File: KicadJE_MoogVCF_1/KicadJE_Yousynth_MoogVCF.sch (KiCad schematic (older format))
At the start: 50 parts

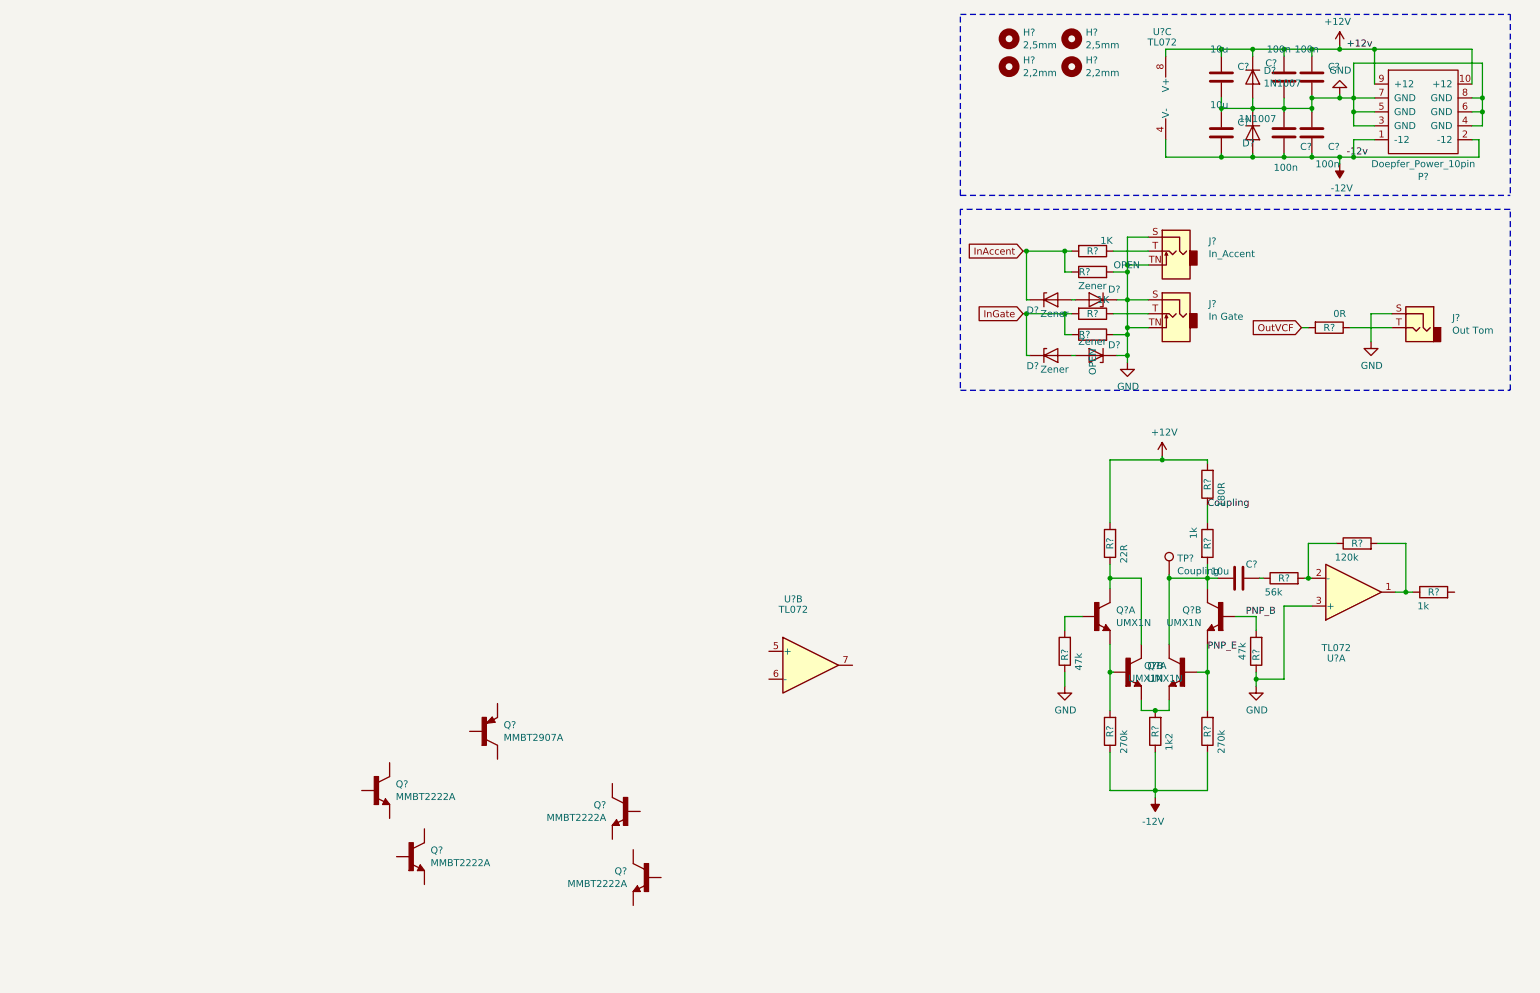
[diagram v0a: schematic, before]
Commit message: Footprints
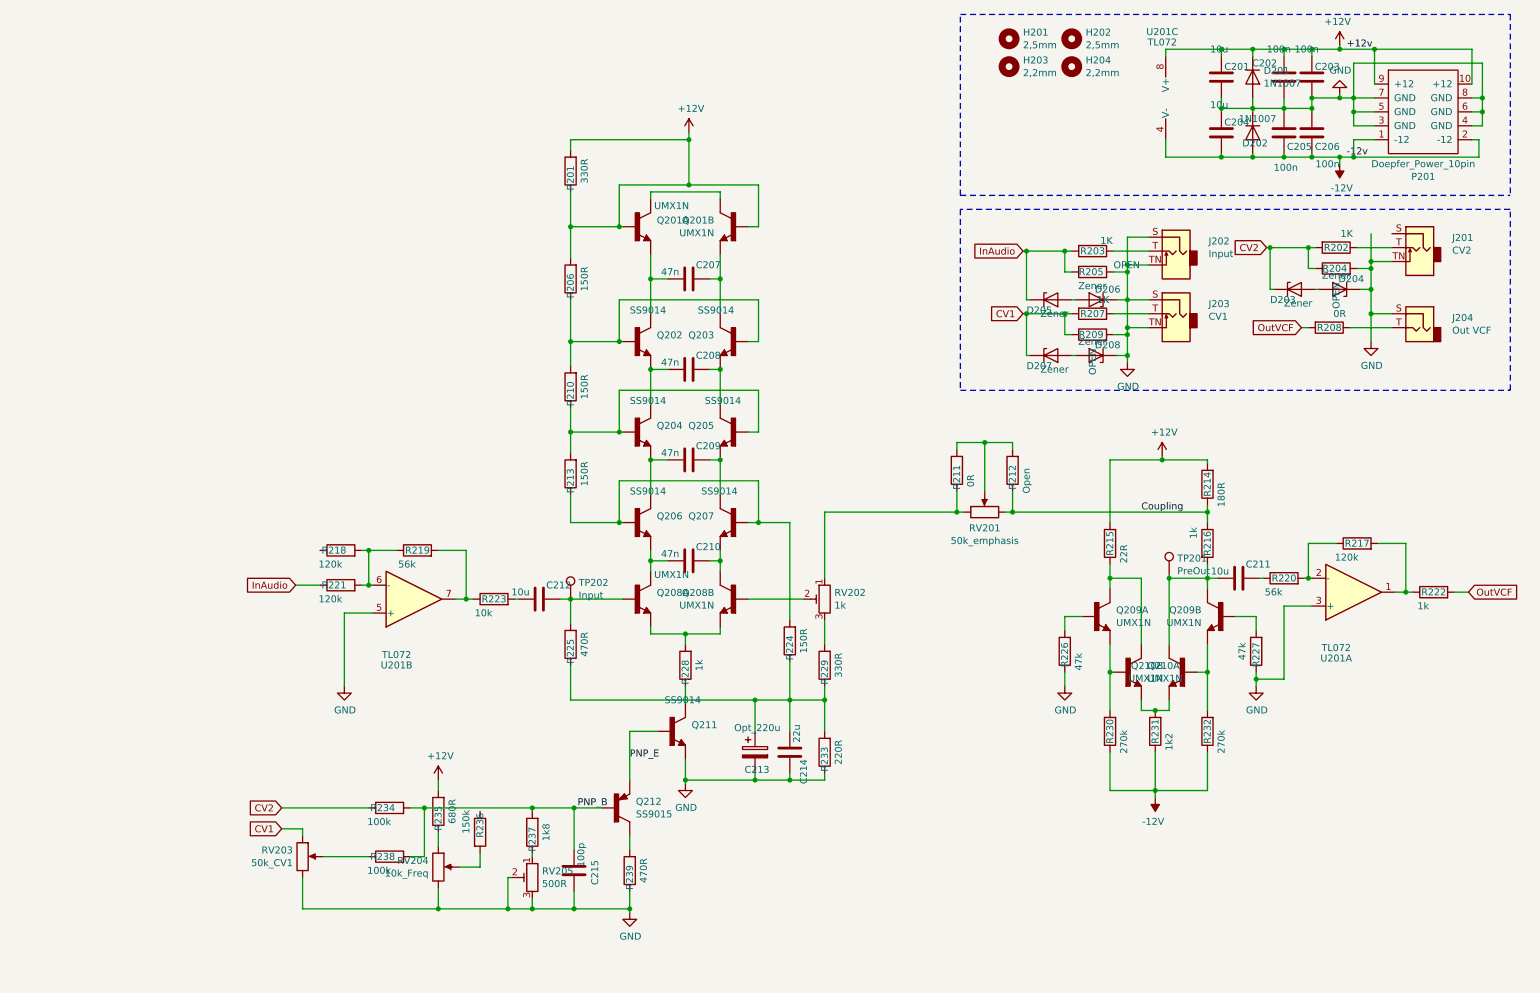
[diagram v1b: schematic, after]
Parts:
- removed Q? (x3): MMBT2222A, Package_TO_SOT_SMD:SOT-23_Handsoldering, symbol MMBT2222A:MMBT2222A
- added C207, C208, C209, C210: 47n, Capacitor_SMD:C_0805_2012Metric_Pad1.15x1.40mm_HandSolder, symbol Device:C
- added C212: 10u, Capacitor_SMD:C_0805_2012Metric_Pad1.15x1.40mm_HandSolder, symbol Device:C
- added C213: Opt_220u, Capacitor_THT:CP_Radial_D10.0mm_P5.00mm, symbol Device:CP
- added C214: 22u, Capacitor_SMD:C_0805_2012Metric_Pad1.15x1.40mm_HandSolder, symbol Device:C
- added C215: 100p, Capacitor_SMD:C_0805_2012Metric_Pad1.15x1.40mm_HandSolder, symbol Device:C
- added D203, D204: Zener, Diode_SMD:D_MiniMELF, symbol Device:D_Zener
- added J201: CV2, AJ-Dropbox-Kicad:PJ301SM, symbol Connector:AudioJack2_SwitchT
- added Q201, Q208: UMX1N, AJ:UMX1N_UMT6_DualNPN, symbol UMX1N:UMX1N
- added Q202, Q203, Q204, Q205, Q207, Q211: SS9014, Package_TO_SOT_SMD:SOT-23_Handsoldering, symbol MMBT2222A:MMBT2222A
- added R201, R229: 330R, Resistor_SMD:R_0805_2012Metric_Pad1.15x1.40mm_HandSolder, symbol Device:R
- added R202: 1K, Resistor_SMD:R_0805_2012Metric_Pad1.15x1.40mm_HandSolder, symbol Device:R
- added R204: OPEN, Resistor_SMD:R_0805_2012Metric_Pad1.15x1.40mm_HandSolder, symbol Device:R
- added R206, R210, R213, R224: 150R, Resistor_SMD:R_0805_2012Metric_Pad1.15x1.40mm_HandSolder, symbol Device:R
- added R211: 0R, Resistor_SMD:R_0805_2012Metric_Pad1.15x1.40mm_HandSolder, symbol Device:R
- added R212: Open, Resistor_SMD:R_0805_2012Metric_Pad1.15x1.40mm_HandSolder, symbol Device:R
- added R218, R221: 120k, Resistor_SMD:R_0805_2012Metric_Pad1.15x1.40mm_HandSolder, symbol Device:R
- added R219: 56k, Resistor_SMD:R_0805_2012Metric_Pad1.15x1.40mm_HandSolder, symbol Device:R
- added R223: 10k, Resistor_SMD:R_0805_2012Metric_Pad1.15x1.40mm_HandSolder, symbol Device:R
- added R225, R239: 470R, Resistor_SMD:R_0805_2012Metric_Pad1.15x1.40mm_HandSolder, symbol Device:R
- added R228: 1k, Resistor_SMD:R_0805_2012Metric_Pad1.15x1.40mm_HandSolder, symbol Device:R
- added R233: 220R, Resistor_SMD:R_0805_2012Metric_Pad1.15x1.40mm_HandSolder, symbol Device:R
- added R234, R238: 100k, Resistor_SMD:R_0805_2012Metric_Pad1.15x1.40mm_HandSolder, symbol Device:R
- added R235: 680R, Resistor_SMD:R_0805_2012Metric_Pad1.15x1.40mm_HandSolder, symbol Device:R
- added R236: 150k, Resistor_SMD:R_0805_2012Metric_Pad1.15x1.40mm_HandSolder, symbol Device:R
- added R237: 1k8, Resistor_SMD:R_0805_2012Metric_Pad1.15x1.40mm_HandSolder, symbol Device:R
- added RV201: 50k_emphasis, AJ-Dropbox-Kicad:Potentiometer_China_RK09_Single_Vertical_AJ, symbol Envelope-cache-2018-08-04-13-00-04:POT
- added RV202: 1k, AJ-Dropbox-Kicad:Bourns3296WV, symbol Device:R_POT_TRIM
- added RV203: 50k_CV1, AJ-Dropbox-Kicad:Potentiometer_China_RK09_Single_Vertical_AJ, symbol Envelope-cache-2018-08-04-13-00-04:POT
- added RV204: 10k_Freq, AJ-Dropbox-Kicad:Potentiometer_China_RK09_Single_Vertical_AJ, symbol Envelope-cache-2018-08-04-13-00-04:POT
- added RV205: 500R, AJ-Dropbox-Kicad:Bourns3296WV, symbol Device:R_POT_TRIM
- added TP202: Input, TestPoint:TestPoint_Pad_1.5x1.5mm, symbol Connector:TestPoint
- J202: renamed from J?; value In_Accent -> Input
- J203: renamed from J?; value In Gate -> CV1
- J204: renamed from J?; value Out Tom -> Out VCF
- Q206: renamed from Q?; value MMBT2222A -> SS9014
- Q209, Q210: renamed from Q?; footprint UMT6 -> AJ:UMX1N_UMT6_DualNPN
- Q212: renamed from Q?; value MMBT2907A -> SS9015
- TP201: renamed from TP?; value Coupling -> PreOut
- gave numbers to parts that had none: 35
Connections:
- net +12V: now also Q201.2 (B), Q201.5 (B), R201.1, R201.2, R206.2, R235.2
- net Coupling: now also R212.1, RV201.3
- net GND: now also U201.5 (+), C213.2, C214.1, C215.1, D204.1 (K), J201.TN, Q211.2 (E), R204.2, R233.1, R239.1, RV203.3, RV204.3, RV205.2, RV205.3
- net OutVCF: now also R222.2
- net PNP_B: now also Q212.1 (B), C215.2, R234.2, R237.2, R238.2; no longer Q209.5 (B), R227.2
- net PNP_E: now also Q212.2 (E), Q211.1 (B); no longer Q209.4 (E), Q210.5 (B), R232.2
- net at Q212.3 (C): now also R239.2
- net at Q206.1 (B): now also Q207.1 (B), R213.1, R224.2
- net at Q206.2 (E): now also C210.2, Q208.6 (C)
- net at Q206.3 (C): now also C209.2, Q204.2 (E)
- net at U201.6 (-): now also R218.2, R219.1, R221.2
- net at U201.7: now also R219.2, R223.1
- net InAccent renamed InAudio
- net InAudio: now also R221.1
- net InGate renamed CV1
- net CV1: now also RV203.1
- new net: Q209.5 (B), R227.2
- new net: Q209.4 (E), Q210.5 (B), R232.2
- new net: J201.T, R202.1
- new net: D203.2 (A), D204.2 (A)
- new net: Q201.3 (C), Q201.6 (C)
- new net: C207.1, Q201.4 (E), Q203.3 (C)
- new net: C207.2, Q201.1 (E), Q202.3 (C)
- new net: C210.1, Q207.2 (E), Q208.3 (C)
- new net: Q208.1 (E), Q208.4 (E), R228.2
- new net: Q208.5 (B), RV202.2
- new net: C212.1, Q208.2 (B), R225.2, TP202.1
- new net: C209.1, Q205.2 (E), Q207.3 (C)
- new net: Q204.1 (B), Q205.1 (B), R210.1, R213.2
- new net: C208.2, Q202.2 (E), Q204.3 (C)
- new net: C208.1, Q203.2 (E), Q205.3 (C)
- new net: Q202.1 (B), Q203.1 (B), R206.1, R210.2
- new net: Q211.3 (C), R228.1
- new net: C213.1, C214.2, R224.1, R225.1, R229.1, R233.2
- new net: R229.2, RV202.3
- new net: R211.1, RV201.1, RV202.1
- new net: R211.2, R212.2, RV201.2
- new net: R237.1, RV205.1
- new net: C212.2, R223.2
- new net: R238.1, RV203.2
- new net: R235.1, RV204.1
- new net: R236.2, RV204.2
- new net CV2: D203.1 (K), R202.2, R204.1, R234.1
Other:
- moved on the sheet: Q206, Q212, U201B

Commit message: Placing components
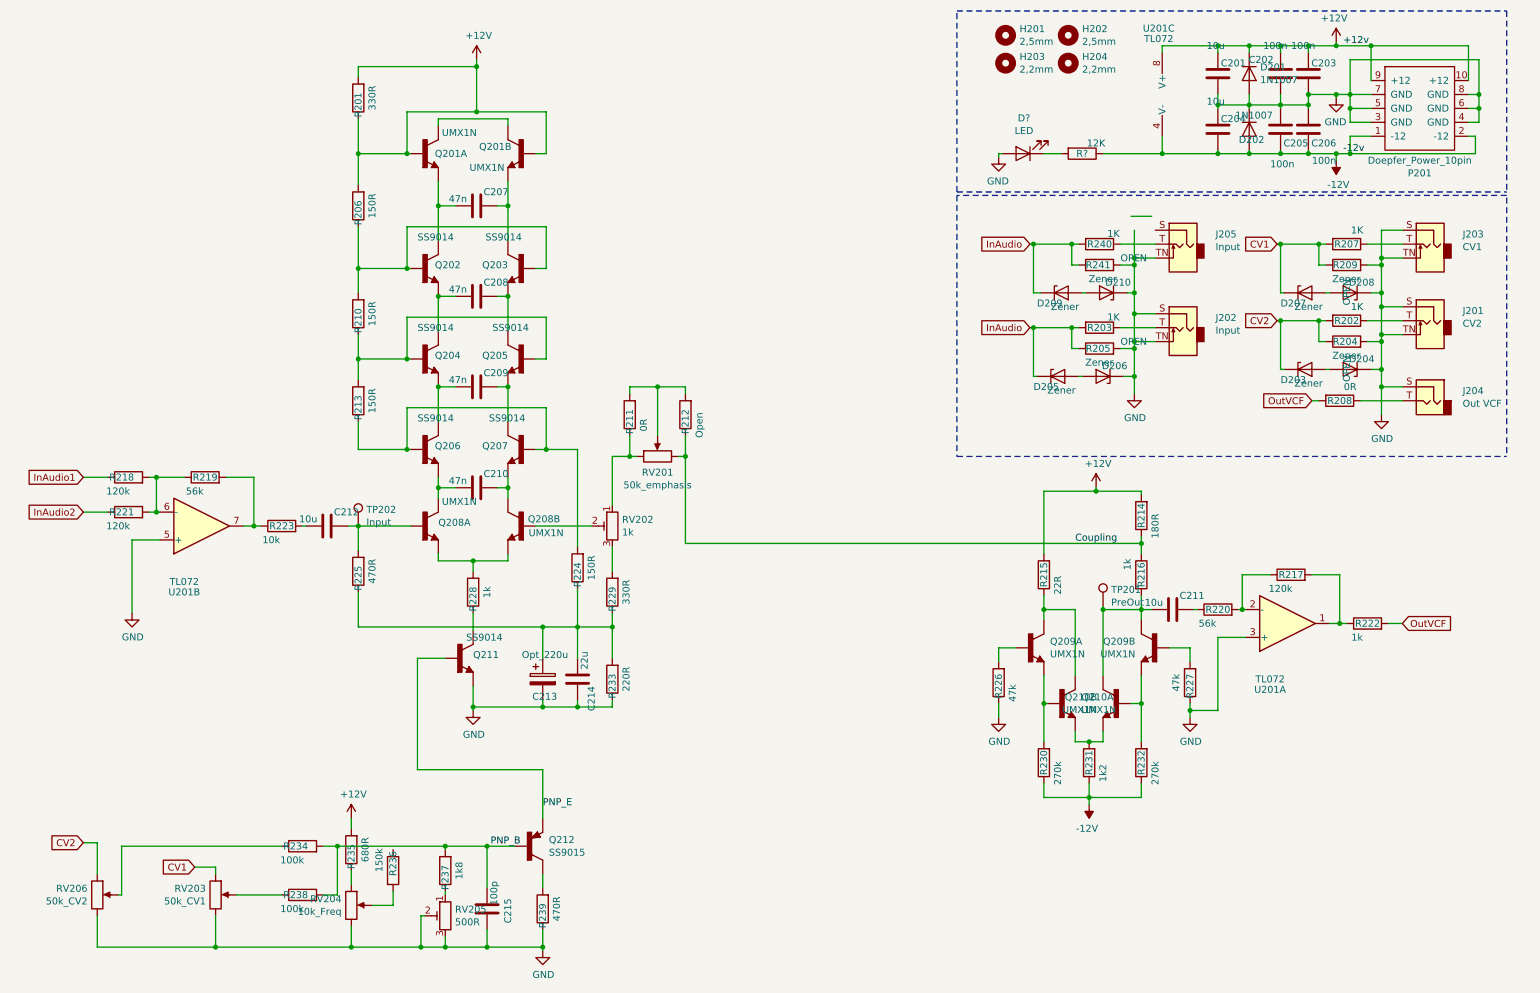
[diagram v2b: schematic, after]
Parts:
- added D209, D210: Zener, Diode_SMD:D_MiniMELF, symbol Device:D_Zener
- added D?: LED, LED_SMD:LED_0805_2012Metric, symbol Device:LED
- added J205: Input, AJ-Dropbox-Kicad:PJ301SM, symbol Connector:AudioJack2_SwitchT
- added R240: 1K, Resistor_SMD:R_0805_2012Metric_Pad1.15x1.40mm_HandSolder, symbol Device:R
- added R241: OPEN, Resistor_SMD:R_0805_2012Metric_Pad1.15x1.40mm_HandSolder, symbol Device:R
- added R?: 12K, Resistor_SMD:R_0805_2012Metric_Pad1.15x1.40mm_HandSolder, symbol Device:R
- added RV206: 50k_CV2, AJ-Dropbox-Kicad:Potentiometer_China_RK09_Single_Vertical_AJ, symbol Envelope-cache-2018-08-04-13-00-04:POT
- J202: footprint Connector_Audio:Jack_3.5mm_Ledino_KB3SPRS_Horizontal -> AJ-Dropbox-Kicad:PJ301SM
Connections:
- net -12V: now also R?.1
- net CV2: now also RV206.1; no longer R234.1
- net GND: now also J201.S, D210.1 (K), D?.2 (A), J205.TN, R241.2, RV206.3
- net InAudio: now also D209.1 (K), R240.2, R241.1; no longer R221.1
- net InAudio1: now reaches R218.1
- new net: R234.1, RV206.2
- new net: J205.T, R240.1
- new net: D209.2 (A), D210.2 (A)
- new net: D?.1 (K), R?.2
- new net InAudio2: R221.1
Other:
- moved on the sheet: C201, C202, C203, C204, C205, C206, C207, C208, C209, C210, C211, C212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
